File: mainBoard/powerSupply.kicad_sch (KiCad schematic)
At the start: 50 parts, among them J1 1366005, SW5 SW_DPST_x2, U1 MCP1727T-3302E/SN, U2 AP62250WU, U3 MCP1727T-3302E/SN

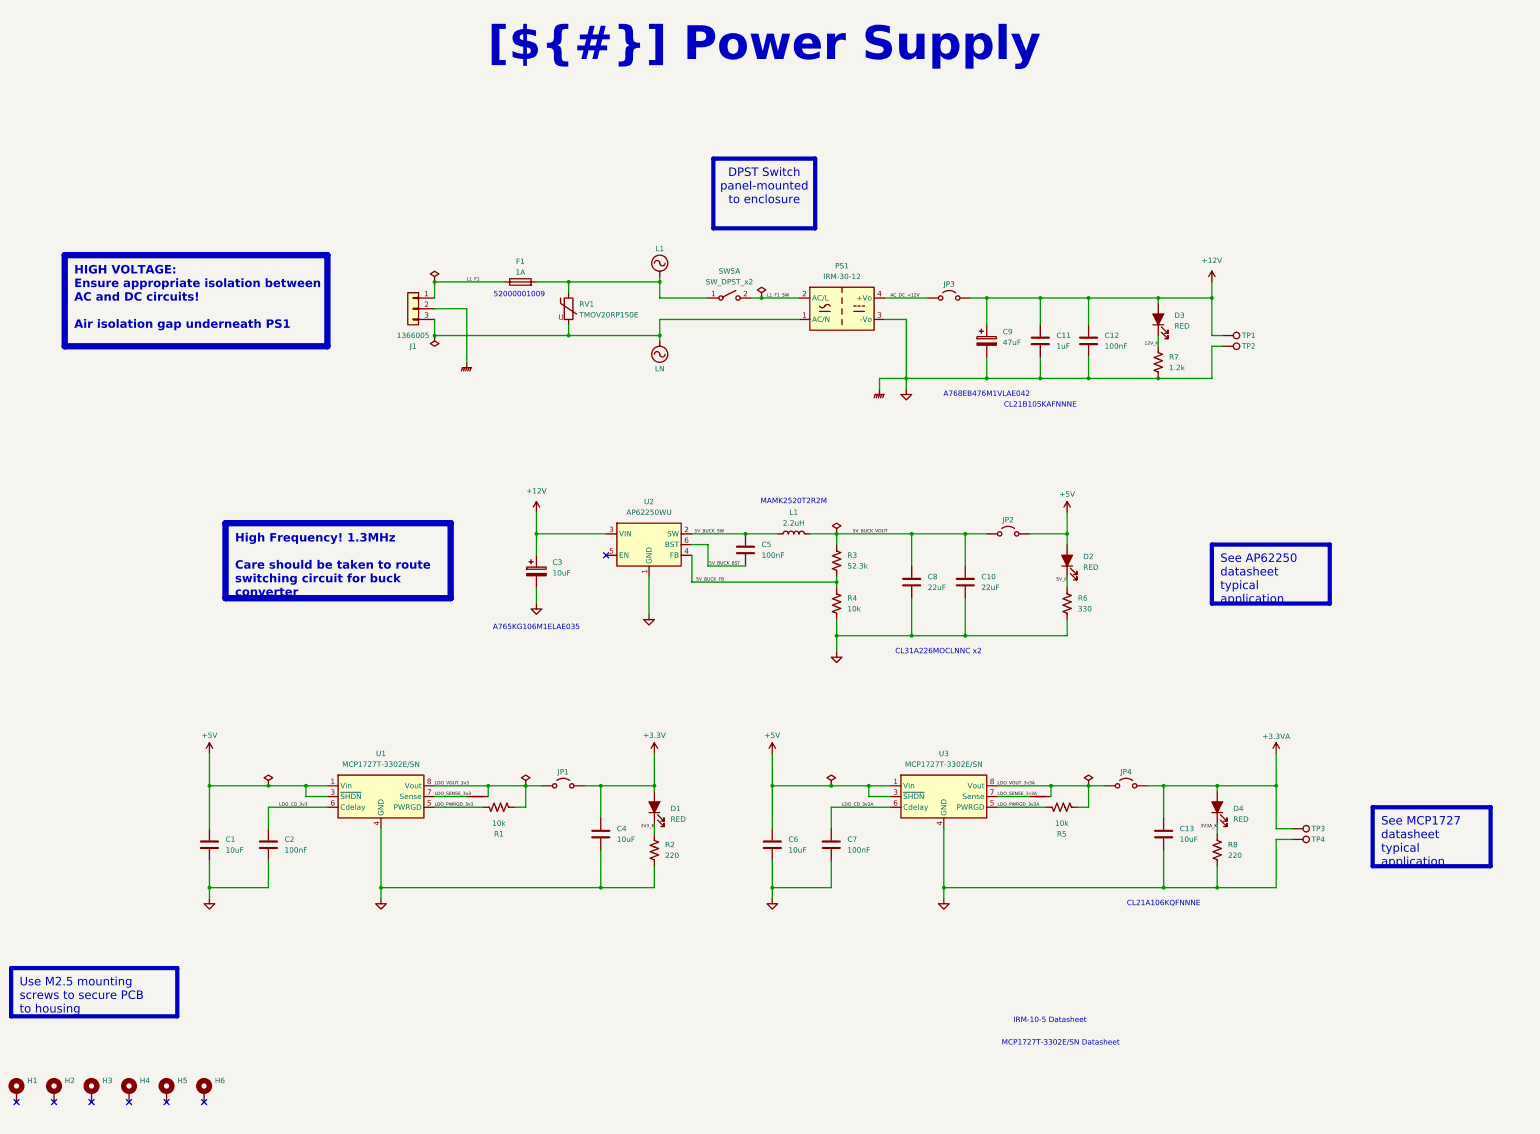
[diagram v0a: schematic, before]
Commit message: Nearly finished with board after revisions
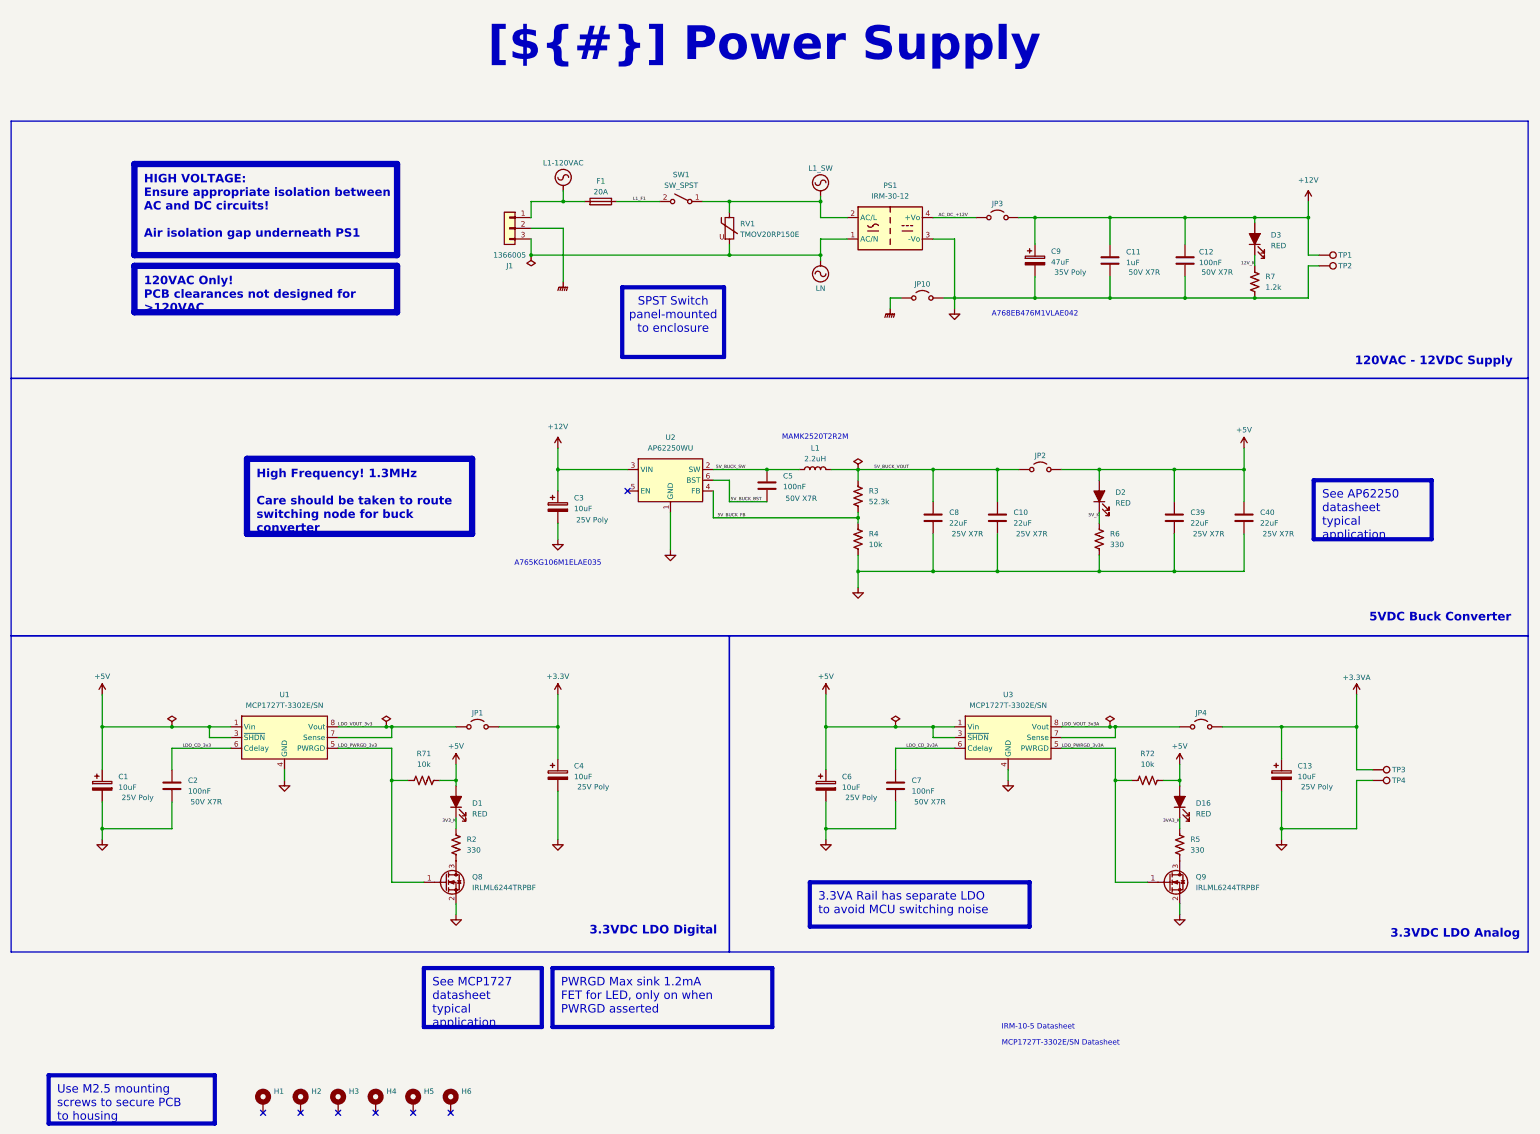
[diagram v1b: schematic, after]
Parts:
- removed C1, C13, C4, C6: 10uF, Capacitor_SMD:C_0805_2012Metric_Pad1.18x1.45mm_HandSolder, symbol Device:C
- removed D4: RED, LED_SMD:LED_0603_1608Metric_Pad1.05x0.95mm_HandSolder, symbol Device:LED_Filled
- removed NT1, NT2: NetTie_2, NetTie:NetTie-2_SMD_Pad0.5mm, symbol Device:NetTie_2
- removed R1: 10k, Resistor_SMD:R_0603_1608Metric_Pad0.98x0.95mm_HandSolder, symbol Device:R_US
- removed R8: 220, Resistor_SMD:R_0603_1608Metric_Pad0.98x0.95mm_HandSolder, symbol Device:R_US
- added C1, C13, C4, C6: 10uF, Capacitor_SMD:C_Elec_6.3x5.8, symbol Device:C_Polarized
- added C39, C40: 22uF, Capacitor_SMD:C_1206_3216Metric_Pad1.33x1.80mm_HandSolder, symbol Device:C
- added D16: RED, LED_SMD:LED_0603_1608Metric_Pad1.05x0.95mm_HandSolder, symbol Device:LED_Filled
- added JP10: Jumper_2_Open, Jumper:SolderJumper-2_P1.3mm_Open_TrianglePad1.0x1.5mm, symbol Jumper:Jumper_2_Open
- added Q8, Q9: IRLML6244TRPBF, Package_TO_SOT_SMD:SOT-23, symbol Transistor_FET:IRLML6244
- added R71, R72: 10k, Resistor_SMD:R_0603_1608Metric_Pad0.98x0.95mm_HandSolder, symbol Device:R_US
- C10, C8: Type (none) -> 25V X7R
- C11, C12, C5: Type (none) -> 50V X7R
- C2, C7: footprint Capacitor_SMD:C_0805_2012Metric_Pad1.18x1.45mm_HandSolder -> Capacitor_SMD:C_0603_1608Metric_Pad1.08x0.95mm_HandSolder; Type (none) -> 50V X7R
- C3: Type (none) -> 25V Poly
- C9: Type (none) -> 35V Poly
- F1: value 1A -> 20A; footprint Fuse:Fuseholder_Clip-5x20mm_Littelfuse_100_Inline_P20.50x4.60mm_D1.30mm_Horizontal -> Fuse:Fuseholder_Clip-6.3x32mm_Littelfuse_122_Inline_P34.21x7.62mm_D2.54mm_Horizontal
- R2: value 220 -> 330
- R5: value 10k -> 330
- SW1: renamed from SW5; value SW_DPST_x2 -> SW_SPST; symbol Switch:SW_DPST_x2 -> Switch:SW_SPST
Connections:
- net LDO_SENSE_3v3 is gone; now on net LDO_VOUT_3v3: U1.7 (Sense)
- net LDO_SENSE_3v3A is gone; now on net LDO_VOUT_3v3A: U3.7 (Sense)
- net +3.3V: now also C4.1; no longer D1.2 (A)
- net +3.3VA: now also C13.1
- net +5V: now also D1.2 (A), C1.1, C39.1, C40.1, C6.1, D16.2 (A), R71.2, R72.2
- net GND: now also C1.2, C13.2, C39.2, C4.2, C40.2, C6.2, JP10.2 (B), Q8.2 (S), Q9.2 (S); no longer J1.2 (Pin_2), R2.2
- net L1_F1: now also SW1.2 (B); no longer J1.1 (Pin_1)
- net LDO_PWRGD_3v3: now also Q8.1 (G), R71.1
- net LDO_PWRGD_3v3A: now also Q9.1 (G), R72.1; no longer R5.2
- net LDO_VOUT_3v3A: no longer R5.1
- net L1 renamed L1_SW
- net L1_SW: now also PS1.2 (AC/L); no longer F1.2
- removed net L1_F1_SW: PS1.2 (AC/L), SW1.2 (B)
- new net: Q9.3 (D), R5.2
- new net: Q8.3 (D), R2.2
- new net 3VA3_K: D16.1 (K), R5.1
- new net GNDPWR: J1.2 (Pin_2), JP10.1 (A)
- new net L1-120VAC: F1.2, J1.1 (Pin_1)
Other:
- note added: "120VAC - 12VDC Supply"
- note added: "3.3VDC LDO Analog"
- note added: "3.3VDC LDO Digital"
- note added: "5VDC Buck Converter"
- note removed: "52000001009"
- note removed: "CL21A106KQFNNNE"
- note removed: "CL21B105KAFNNNE"
- note removed: "CL31A226MOCLNNC x2"
- moved on the sheet: C10, C11, C12, C2, C3, C5, C8, C9, D1, D2, D3, H1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
